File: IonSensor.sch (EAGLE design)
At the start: 20 parts, among them IC1 QUAD_OPAMPD, IC2 QUAD_OPAMPD, IC3 QUAD_OPAMPD, X1 JST-XH-04-PIN-LONG-PAD

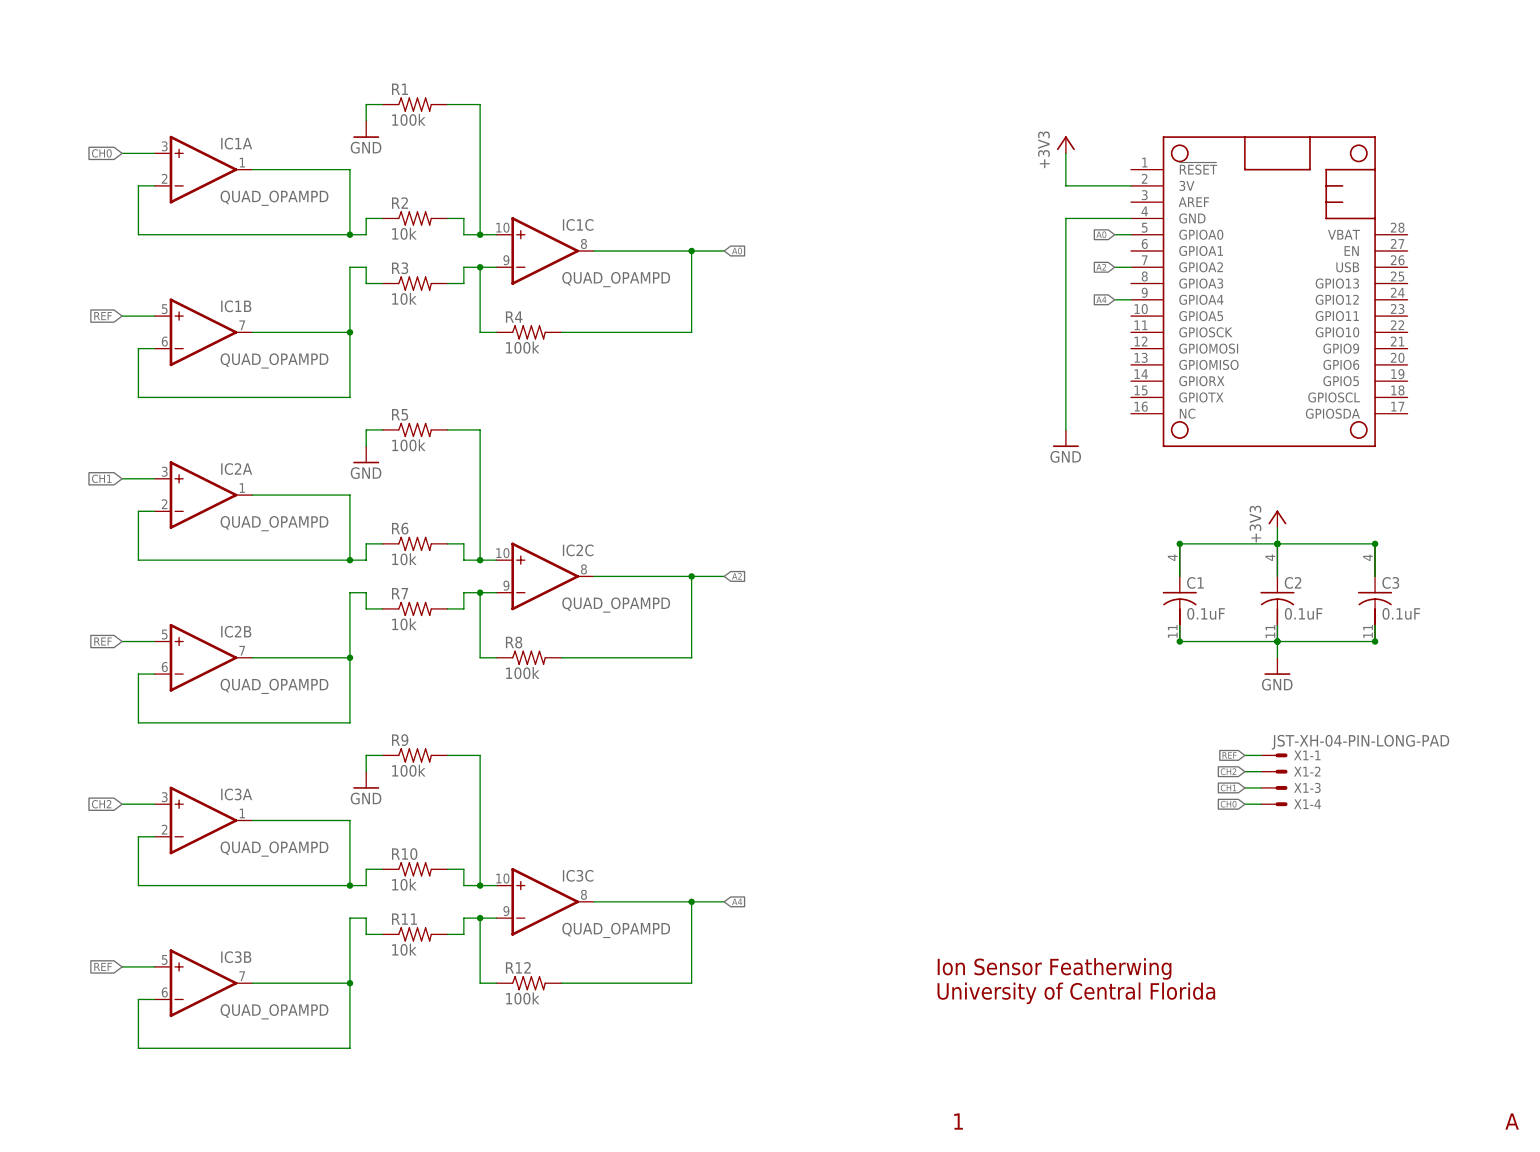
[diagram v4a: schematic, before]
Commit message: Revert "Fixed wiring"
This reverts commit 887158206b74e515af25e9af216689274ec85624.
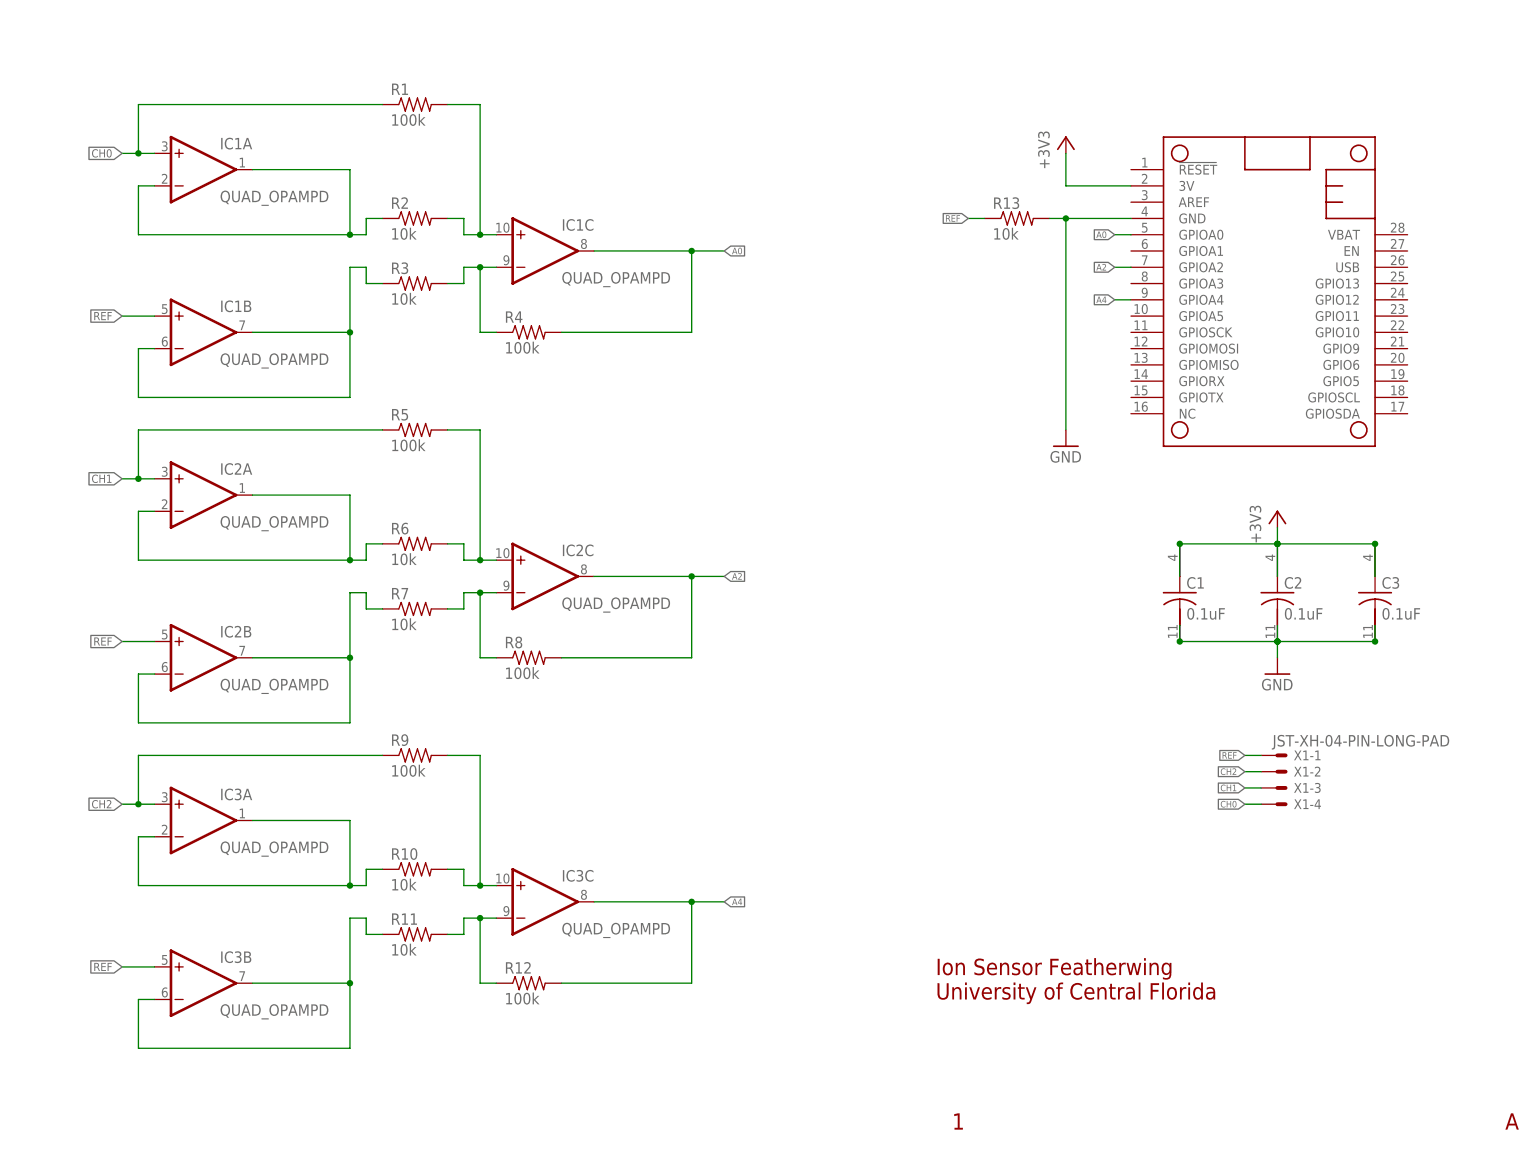
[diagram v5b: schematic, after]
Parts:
- added R13: 10k, rcl:R-US_R0603
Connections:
- net CH0: now also R1.1
- net CH1: now also R5.1
- net CH2: now also R9.1
- net GND: now also R13.2; no longer R1.1, R5.1, R9.1
- net REF: now also R13.1
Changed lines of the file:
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@@
 <part name="+3V1" library="supply1" library_urn="urn:adsk.eagle:library:371" deviceset="+3V3" device=""/>
 <part name="X1" library="Rembrandt Electronics - JST XH Connectors v1-0" deviceset="JST-XH-04-PIN" device="-LONG-PAD"/>
-<part name="GND1" library="supply1" library_urn="urn:adsk.eagle:library:371" deviceset="GND" device=""/>
-<part name="GND2" library="supply1" library_urn="urn:adsk.eagle:library:371" deviceset="GND" device=""/>
-<part name="GND3" library="supply1" library_urn="urn:adsk.eagle:library:371" deviceset="GND" device=""/>
+<part name="R13" library="rcl" library_urn="urn:adsk.eagle:library:334" deviceset="R-US_" device="R0603" package3d_urn="urn:adsk.eagle:package:23555/3" value="10k"/>
 </parts>
 <sheets>
@@
 <attribute name="NAME" x="205.74" y="57.658" size="1.524" layer="95"/>
 </instance>
-<instance part="GND1" gate="1" x="60.96" y="162.56" smashed="yes">
-<attribute name="VALUE" x="58.42" y="160.02" size="1.778" layer="96"/>
-</instance>
-<instance part="GND2" gate="1" x="60.96" y="111.76" smashed="yes">
-<attribute name="VALUE" x="58.42" y="109.22" size="1.778" layer="96"/>
-</instance>
-<instance part="GND3" gate="1" x="60.96" y="60.96" smashed="yes">
-<attribute name="VALUE" x="58.42" y="58.42" size="1.778" layer="96"/>
+<instance part="R13" gate="G$1" x="162.56" y="149.86" smashed="yes">
+<attribute name="NAME" x="158.75" y="151.3586" size="1.778" layer="95"/>
+<attribute name="VALUE" x="158.75" y="146.558" size="1.778" layer="96"/>
 </instance>
 </instances>
@@
 <wire x1="170.18" y1="116.84" x2="170.18" y2="149.86" width="0.1524" layer="91"/>
 <wire x1="170.18" y1="149.86" x2="180.34" y2="149.86" width="0.1524" layer="91"/>
+<pinref part="R13" gate="G$1" pin="2"/>
+<wire x1="170.18" y1="149.86" x2="167.64" y2="149.86" width="0.1524" layer="91"/>
+<junction x="170.18" y="149.86"/>
 </segment>
 <segment>
@@
 <junction x="187.96" y="83.82"/>
 </segment>
-<segment>
-<pinref part="GND1" gate="1" pin="GND"/>
-<wire x1="60.96" y1="165.1" x2="60.96" y2="167.64" width="0.1524" layer="91"/>
-<pinref part="R1" gate="G$1" pin="1"/>
-<wire x1="60.96" y1="167.64" x2="63.5" y2="167.64" width="0.1524" layer="91"/>
-</segment>
-<segment>
-<pinref part="GND2" gate="1" pin="GND"/>
-<wire x1="60.96" y1="114.3" x2="60.96" y2="116.84" width="0.1524" layer="91"/>
-<pinref part="R5" gate="G$1" pin="1"/>
-<wire x1="60.96" y1="116.84" x2="63.5" y2="116.84" width="0.1524" layer="91"/>
-</segment>
-<segment>
-<pinref part="GND3" gate="1" pin="GND"/>
-<wire x1="60.96" y1="63.5" x2="60.96" y2="66.04" width="0.1524" layer="91"/>
-<pinref part="R9" gate="G$1" pin="1"/>
-<wire x1="60.96" y1="66.04" x2="63.5" y2="66.04" width="0.1524" layer="91"/>
-</segment>
 </net>
 <net name="+3V3" class="0">
@@
 <segment>
 <pinref part="IC1" gate="A" pin="+IN"/>
+<wire x1="22.86" y1="160.02" x2="25.4" y2="160.02" width="0.1524" layer="91"/>
 <label x="22.86" y="160.02" size="1.27" layer="95" rot="R180" xref="yes"/>
-<wire x1="22.86" y1="160.02" x2="27.94" y2="160.02" width="0.1524" layer="91"/>
+<pinref part="R1" gate="G$1" pin="1"/>
+<wire x1="25.4" y1="160.02" x2="27.94" y2="160.02" width="0.1524" layer="91"/>
+<wire x1="63.5" y1="167.64" x2="25.4" y2="167.64" width="0.1524" layer="91"/>
+<wire x1="25.4" y1="167.64" x2="25.4" y2="160.02" width="0.1524" layer="91"/>
+<junction x="25.4" y="160.02"/>
 </segment>
 <segment>
@@
 <label x="22.86" y="83.82" size="1.27" layer="95" rot="R180" xref="yes"/>
 <pinref part="IC2" gate="B" pin="+IN"/>
+</segment>
+<segment>
+<pinref part="R13" gate="G$1" pin="1"/>
+<wire x1="154.94" y1="149.86" x2="157.48" y2="149.86" width="0.1524" layer="91"/>
+<label x="154.94" y="149.86" size="1.016" layer="95" rot="R180" xref="yes"/>
 </segment>
 <segment>
@@
 <segment>
 <pinref part="IC2" gate="A" pin="+IN"/>
+<wire x1="22.86" y1="109.22" x2="25.4" y2="109.22" width="0.1524" layer="91"/>
 <label x="22.86" y="109.22" size="1.27" layer="95" rot="R180" xref="yes"/>
-<wire x1="22.86" y1="109.22" x2="27.94" y2="109.22" width="0.1524" layer="91"/>
+<pinref part="R5" gate="G$1" pin="1"/>
+<wire x1="25.4" y1="109.22" x2="27.94" y2="109.22" width="0.1524" layer="91"/>
+<wire x1="63.5" y1="116.84" x2="25.4" y2="116.84" width="0.1524" layer="91"/>
+<wire x1="25.4" y1="116.84" x2="25.4" y2="109.22" width="0.1524" layer="91"/>
+<junction x="25.4" y="109.22"/>
 </segment>
 <segment>
@@
 <segment>
 <pinref part="IC3" gate="A" pin="+IN"/>
+<wire x1="22.86" y1="58.42" x2="25.4" y2="58.42" width="0.1524" layer="91"/>
 <label x="22.86" y="58.42" size="1.27" layer="95" rot="R180" xref="yes"/>
-<wire x1="22.86" y1="58.42" x2="27.94" y2="58.42" width="0.1524" layer="91"/>
+<pinref part="R9" gate="G$1" pin="1"/>
+<wire x1="25.4" y1="58.42" x2="27.94" y2="58.42" width="0.1524" layer="91"/>
+<wire x1="63.5" y1="66.04" x2="25.4" y2="66.04" width="0.1524" layer="91"/>
+<wire x1="25.4" y1="66.04" x2="25.4" y2="58.42" width="0.1524" layer="91"/>
+<junction x="25.4" y="58.42"/>
 </segment>
 <segment>
@@
 packages will not be understood (or retained) with this version.
 </note>
+<note version="8.4" severity="warning">
+Since Version 8.4, EAGLE supports properties for SPICE simulation.
+Probes in schematics and SPICE mapping objects found in parts and library devices
+will not be understood with this version. Update EAGLE to the latest version
+for full support of SPICE simulation.
+</note>
 </compatibility>

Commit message: Fixed wiring
Made sure it's a differential amplifier!
Removed R13.
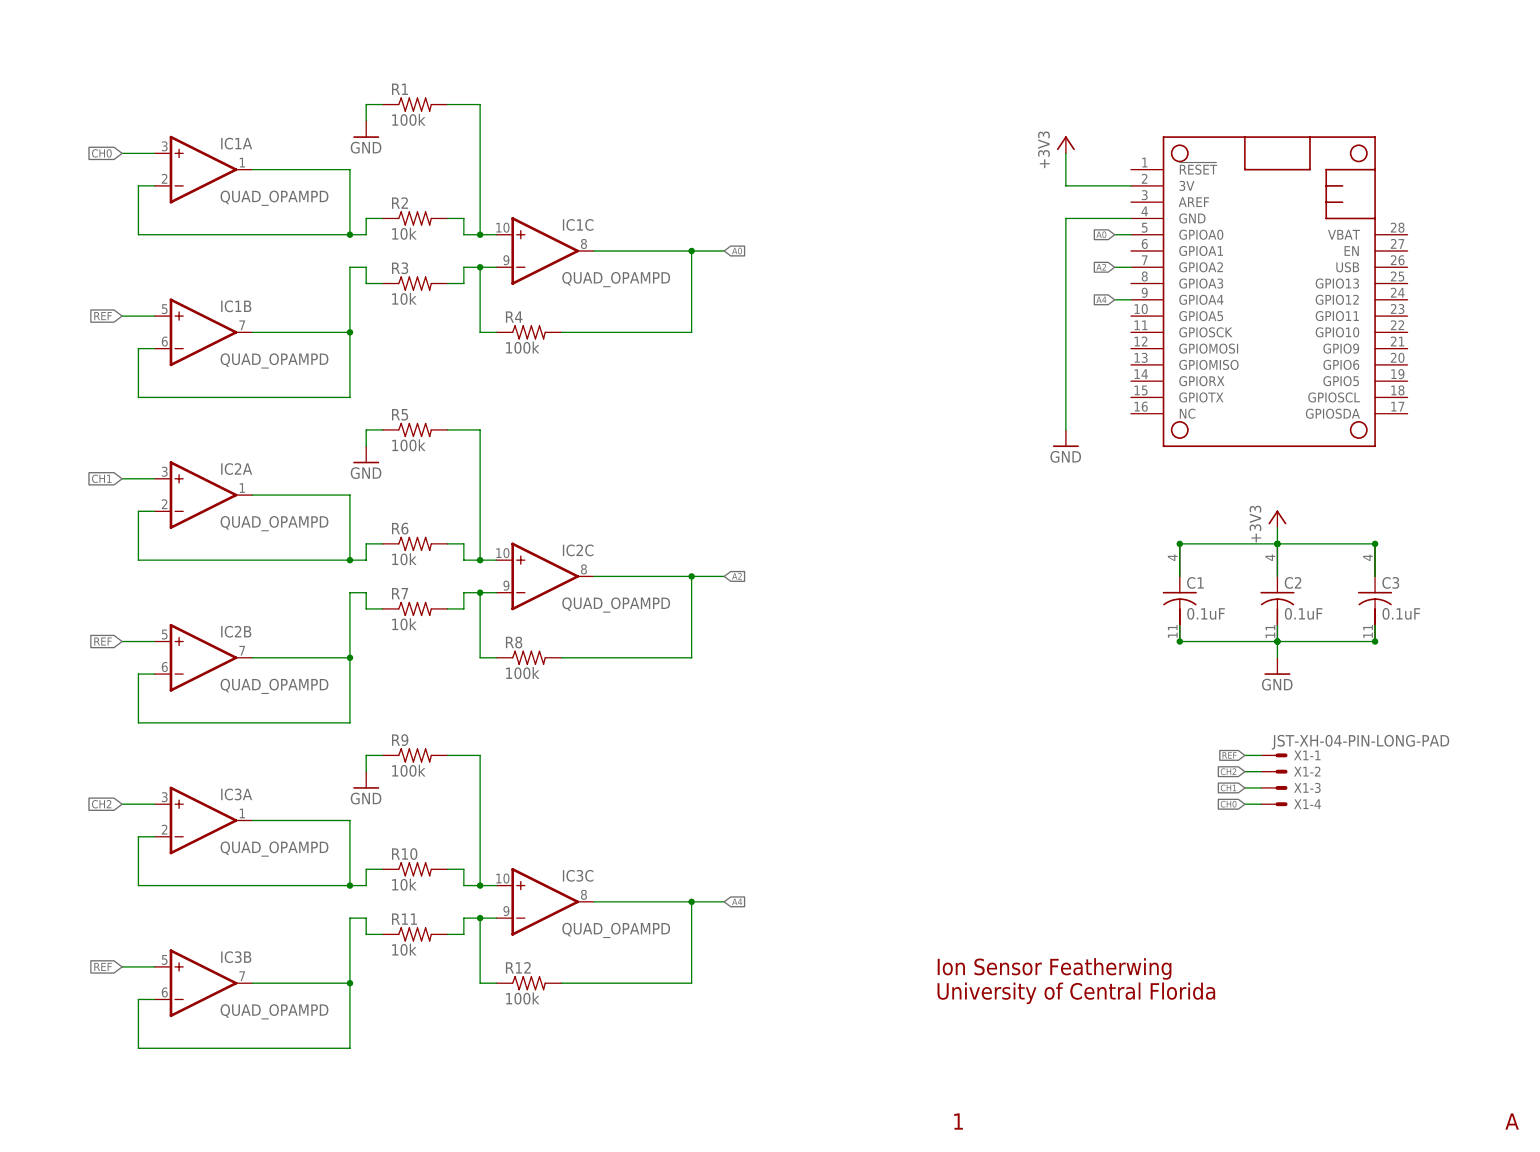
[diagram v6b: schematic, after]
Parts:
- removed R13: 10k, rcl:R-US_R0603
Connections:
- net CH0: no longer R1.1
- net CH1: no longer R5.1
- net CH2: no longer R9.1
- net GND: now also R1.1, R5.1, R9.1; no longer R13.2
- net REF: no longer R13.1
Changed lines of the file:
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@@
 <part name="+3V1" library="supply1" library_urn="urn:adsk.eagle:library:371" deviceset="+3V3" device=""/>
 <part name="X1" library="Rembrandt Electronics - JST XH Connectors v1-0" deviceset="JST-XH-04-PIN" device="-LONG-PAD"/>
-<part name="R13" library="rcl" library_urn="urn:adsk.eagle:library:334" deviceset="R-US_" device="R0603" package3d_urn="urn:adsk.eagle:package:23555/3" value="10k"/>
+<part name="GND1" library="supply1" library_urn="urn:adsk.eagle:library:371" deviceset="GND" device=""/>
+<part name="GND2" library="supply1" library_urn="urn:adsk.eagle:library:371" deviceset="GND" device=""/>
+<part name="GND3" library="supply1" library_urn="urn:adsk.eagle:library:371" deviceset="GND" device=""/>
 </parts>
 <sheets>
@@
 <attribute name="NAME" x="205.74" y="57.658" size="1.524" layer="95"/>
 </instance>
-<instance part="R13" gate="G$1" x="162.56" y="149.86" smashed="yes">
-<attribute name="NAME" x="158.75" y="151.3586" size="1.778" layer="95"/>
-<attribute name="VALUE" x="158.75" y="146.558" size="1.778" layer="96"/>
+<instance part="GND1" gate="1" x="60.96" y="162.56" smashed="yes">
+<attribute name="VALUE" x="58.42" y="160.02" size="1.778" layer="96"/>
+</instance>
+<instance part="GND2" gate="1" x="60.96" y="111.76" smashed="yes">
+<attribute name="VALUE" x="58.42" y="109.22" size="1.778" layer="96"/>
+</instance>
+<instance part="GND3" gate="1" x="60.96" y="60.96" smashed="yes">
+<attribute name="VALUE" x="58.42" y="58.42" size="1.778" layer="96"/>
 </instance>
 </instances>
@@
 <wire x1="170.18" y1="116.84" x2="170.18" y2="149.86" width="0.1524" layer="91"/>
 <wire x1="170.18" y1="149.86" x2="180.34" y2="149.86" width="0.1524" layer="91"/>
-<pinref part="R13" gate="G$1" pin="2"/>
-<wire x1="170.18" y1="149.86" x2="167.64" y2="149.86" width="0.1524" layer="91"/>
-<junction x="170.18" y="149.86"/>
 </segment>
 <segment>
@@
 <junction x="187.96" y="83.82"/>
 </segment>
+<segment>
+<pinref part="GND1" gate="1" pin="GND"/>
+<wire x1="60.96" y1="165.1" x2="60.96" y2="167.64" width="0.1524" layer="91"/>
+<pinref part="R1" gate="G$1" pin="1"/>
+<wire x1="60.96" y1="167.64" x2="63.5" y2="167.64" width="0.1524" layer="91"/>
+</segment>
+<segment>
+<pinref part="GND2" gate="1" pin="GND"/>
+<wire x1="60.96" y1="114.3" x2="60.96" y2="116.84" width="0.1524" layer="91"/>
+<pinref part="R5" gate="G$1" pin="1"/>
+<wire x1="60.96" y1="116.84" x2="63.5" y2="116.84" width="0.1524" layer="91"/>
+</segment>
+<segment>
+<pinref part="GND3" gate="1" pin="GND"/>
+<wire x1="60.96" y1="63.5" x2="60.96" y2="66.04" width="0.1524" layer="91"/>
+<pinref part="R9" gate="G$1" pin="1"/>
+<wire x1="60.96" y1="66.04" x2="63.5" y2="66.04" width="0.1524" layer="91"/>
+</segment>
 </net>
 <net name="+3V3" class="0">
@@
 <segment>
 <pinref part="IC1" gate="A" pin="+IN"/>
-<wire x1="22.86" y1="160.02" x2="25.4" y2="160.02" width="0.1524" layer="91"/>
 <label x="22.86" y="160.02" size="1.27" layer="95" rot="R180" xref="yes"/>
-<pinref part="R1" gate="G$1" pin="1"/>
-<wire x1="25.4" y1="160.02" x2="27.94" y2="160.02" width="0.1524" layer="91"/>
-<wire x1="63.5" y1="167.64" x2="25.4" y2="167.64" width="0.1524" layer="91"/>
-<wire x1="25.4" y1="167.64" x2="25.4" y2="160.02" width="0.1524" layer="91"/>
-<junction x="25.4" y="160.02"/>
+<wire x1="22.86" y1="160.02" x2="27.94" y2="160.02" width="0.1524" layer="91"/>
 </segment>
 <segment>
@@
 <label x="22.86" y="83.82" size="1.27" layer="95" rot="R180" xref="yes"/>
 <pinref part="IC2" gate="B" pin="+IN"/>
-</segment>
-<segment>
-<pinref part="R13" gate="G$1" pin="1"/>
-<wire x1="154.94" y1="149.86" x2="157.48" y2="149.86" width="0.1524" layer="91"/>
-<label x="154.94" y="149.86" size="1.016" layer="95" rot="R180" xref="yes"/>
 </segment>
 <segment>
@@
 <segment>
 <pinref part="IC2" gate="A" pin="+IN"/>
-<wire x1="22.86" y1="109.22" x2="25.4" y2="109.22" width="0.1524" layer="91"/>
 <label x="22.86" y="109.22" size="1.27" layer="95" rot="R180" xref="yes"/>
-<pinref part="R5" gate="G$1" pin="1"/>
-<wire x1="25.4" y1="109.22" x2="27.94" y2="109.22" width="0.1524" layer="91"/>
-<wire x1="63.5" y1="116.84" x2="25.4" y2="116.84" width="0.1524" layer="91"/>
-<wire x1="25.4" y1="116.84" x2="25.4" y2="109.22" width="0.1524" layer="91"/>
-<junction x="25.4" y="109.22"/>
+<wire x1="22.86" y1="109.22" x2="27.94" y2="109.22" width="0.1524" layer="91"/>
 </segment>
 <segment>
@@
 <segment>
 <pinref part="IC3" gate="A" pin="+IN"/>
-<wire x1="22.86" y1="58.42" x2="25.4" y2="58.42" width="0.1524" layer="91"/>
 <label x="22.86" y="58.42" size="1.27" layer="95" rot="R180" xref="yes"/>
-<pinref part="R9" gate="G$1" pin="1"/>
-<wire x1="25.4" y1="58.42" x2="27.94" y2="58.42" width="0.1524" layer="91"/>
-<wire x1="63.5" y1="66.04" x2="25.4" y2="66.04" width="0.1524" layer="91"/>
-<wire x1="25.4" y1="66.04" x2="25.4" y2="58.42" width="0.1524" layer="91"/>
-<junction x="25.4" y="58.42"/>
+<wire x1="22.86" y1="58.42" x2="27.94" y2="58.42" width="0.1524" layer="91"/>
 </segment>
 <segment>
@@
 packages will not be understood (or retained) with this version.
 </note>
-<note version="8.4" severity="warning">
-Since Version 8.4, EAGLE supports properties for SPICE simulation.
-Probes in schematics and SPICE mapping objects found in parts and library devices
-will not be understood with this version. Update EAGLE to the latest version
-for full support of SPICE simulation.
-</note>
 </compatibility>
